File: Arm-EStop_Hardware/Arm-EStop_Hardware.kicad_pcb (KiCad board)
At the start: 2 copper layers, 24 parts, among them Q1 IRFS7437TRLPBFCT, Q2 IRFS7437TRLPBFCT, SW1 SW_Push_Open, U1 3.3V, U2 LT1910, U3 LT1910, U4 E_STOP, U5 E_STOP+LED

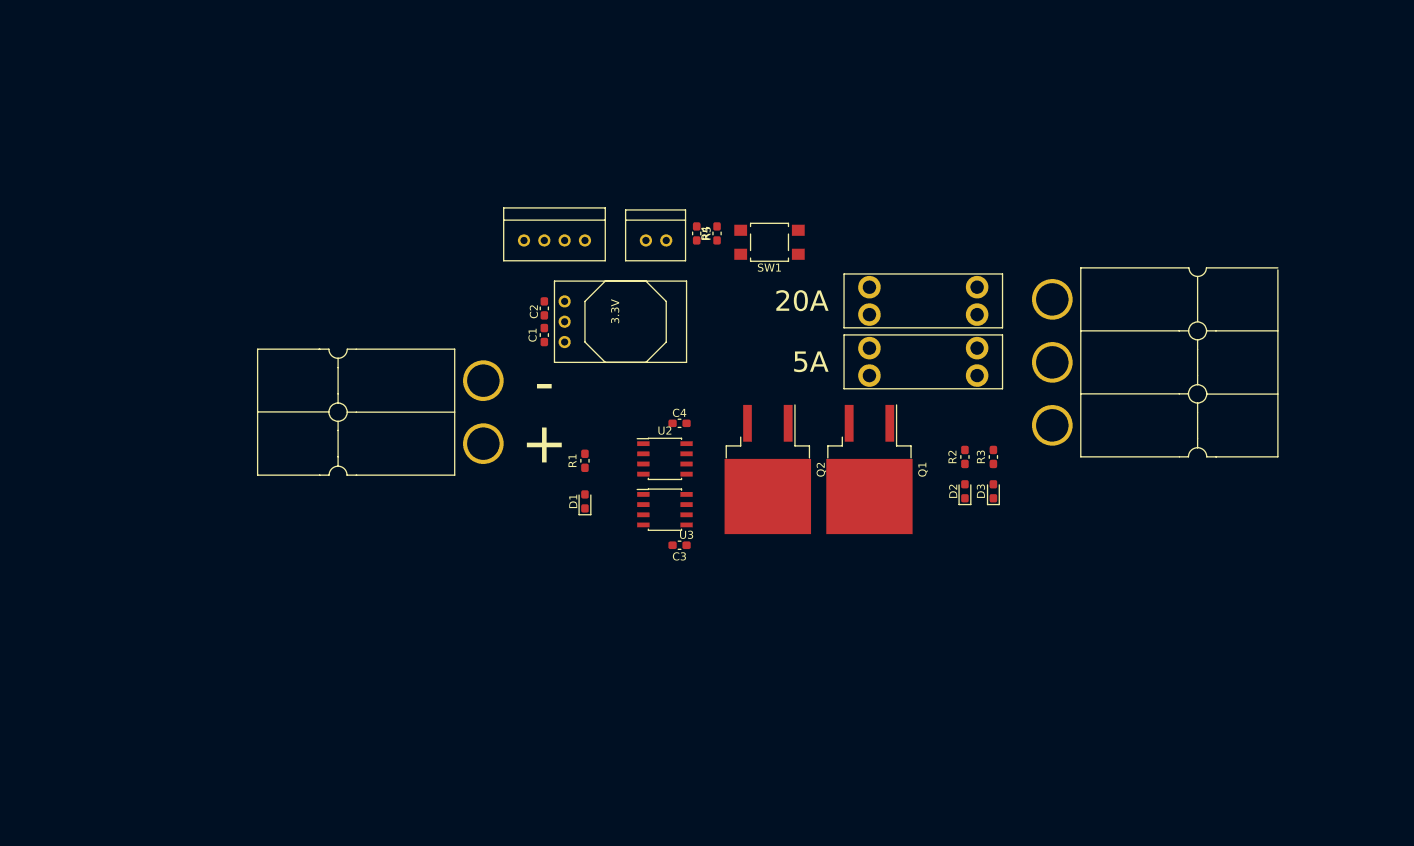
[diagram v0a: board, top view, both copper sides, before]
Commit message: finished layout
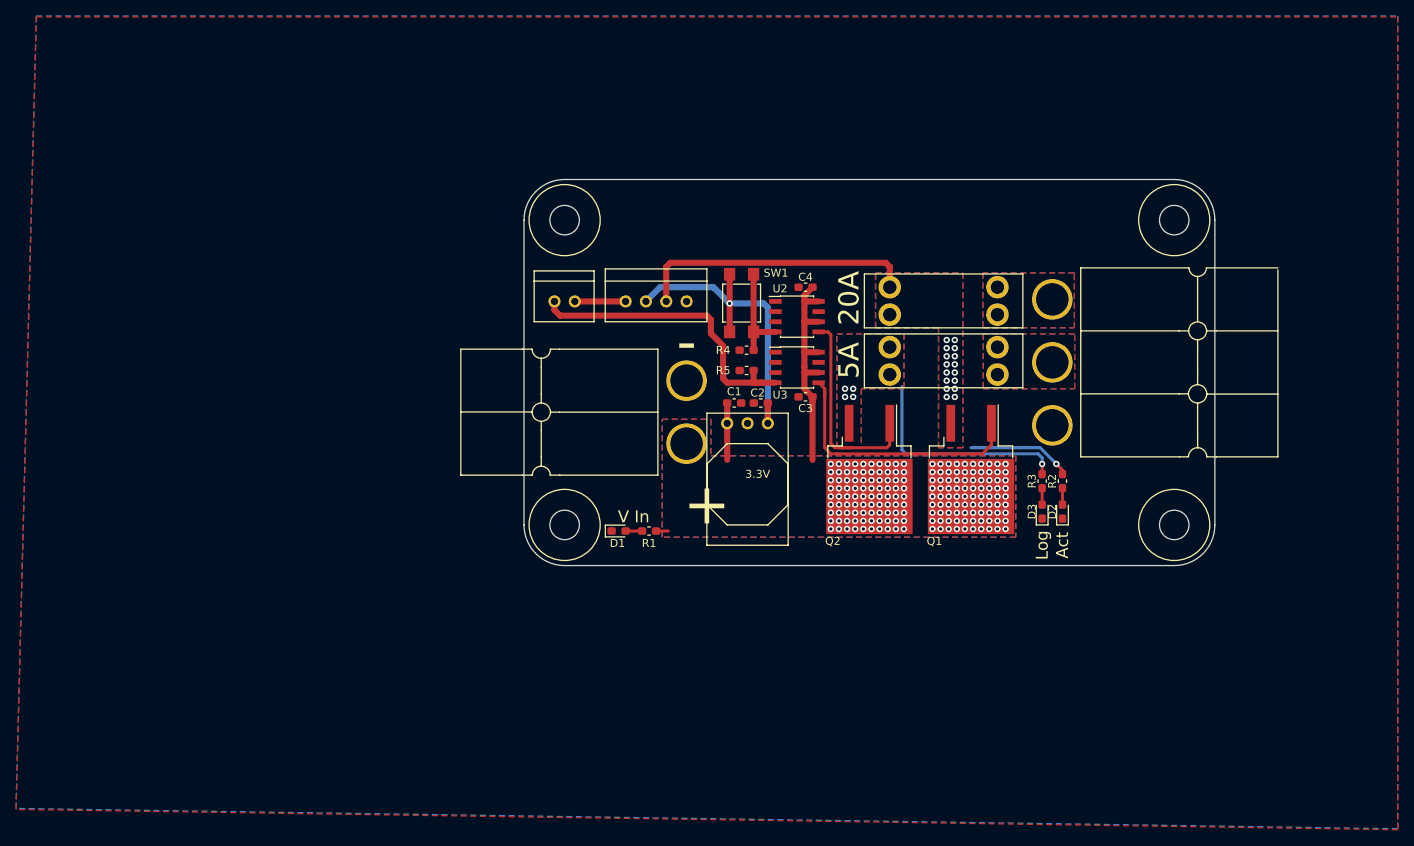
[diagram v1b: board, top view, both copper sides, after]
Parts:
- added REF**: 6_32_Hole, MRDT_Drill_Holes:6_32_Hole_Corner, F.Cu at (214.0, 95.9)
- added REF**: 6_32_Hole, MRDT_Drill_Holes:6_32_Hole_Corner, F.Cu at (146.7, 95.9)
- added REF**: 6_32_Hole, MRDT_Drill_Holes:6_32_Hole_Corner, F.Cu at (146.7, 125.1)
- added REF**: 6_32_Hole, MRDT_Drill_Holes:6_32_Hole_Corner, F.Cu at (214.0, 125.1)
- moved C2 29.5 mm to (166.8, 114.3), turned to 180 degrees
- moved Conn1 25.4 mm to (153.9, 123.3)
- moved C1 25.2 mm to (163.4, 114.3), turned to 0 degrees
- moved C3 24.3 mm to (172.4, 113.5)
- moved U2 24.3 mm to (171.3, 103.5)
- moved U3 24.3 mm to (171.3, 109.9)
- moved C4 23.2 mm to (172.4, 99.8)
- moved U1 20.1 mm to (160.0, 115.6), turned to 0 degrees
- moved R5 18.2 mm to (165.0, 110.2), turned to 180 degrees
- moved R4 15.1 mm to (165.0, 107.7), turned to 180 degrees
- moved U5 14.8 mm to (153.7, 101.6)
- moved U4 13.7 mm to (142.2, 101.6)
- moved Q2 12.7 mm to (180.3, 122.6)
- moved Q1 12.7 mm to (193.0, 122.6)
- moved R2 12.6 mm to (204.5, 124.1)
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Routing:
- net V_Out_Act: track 0.00 -> 48.3 mm, vias 0 -> 17
- net +3V3: track 0.00 -> 41.2 mm, vias 0 -> 1
- net Net-(R5-Pad1): track 0.00 -> 38.4 mm
- net V_In: track 0.00 -> 38.2 mm, vias 0 -> 180
- net E-Stop_Gate: track 0.00 -> 33.5 mm
- net V_Out_Log: track 0.00 -> 27.9 mm, vias 0 -> 5
- net V_Log_Gate: track 0.00 -> 27.2 mm
- net Net-(R4-Pad1): track 0.00 -> 12.2 mm
- net Net-(U4-Pad2): track 0.00 -> 6.35 mm
- net Net-(D3-Pad2): track 0.00 -> 2.06 mm
- net Net-(D2-Pad2): track 0.00 -> 2.06 mm
- net Net-(D1-Pad2): track 0.00 -> 2.06 mm
- added copper zone on B.Cu, net GND
- added copper zone on F.Cu, net GND
- added copper zone on B.Cu, net Net-(Conn2-Pad2)
- added copper zone on F.Cu, net Net-(Conn2-Pad2)
- added copper zone on B.Cu, net Net-(Conn2-Pad3)
- added copper zone on F.Cu, net Net-(Conn2-Pad3)
- added copper zone on B.Cu, net V_In
- added copper zone on F.Cu, net V_In
- added copper zone on B.Cu, net V_Out_Act
- added copper zone on F.Cu, net V_Out_Act
- added copper zone on B.Cu, net V_Out_Log
- added copper zone on F.Cu, net V_Out_Log
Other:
- board outline added: 86.4 x 48.3 mm
- board text added: "Act"
- board text added: "Log"
- board text added: "V In"
